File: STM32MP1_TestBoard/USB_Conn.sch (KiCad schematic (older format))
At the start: 4 parts, among them J13 USB_B_Micro, J14 USB_B

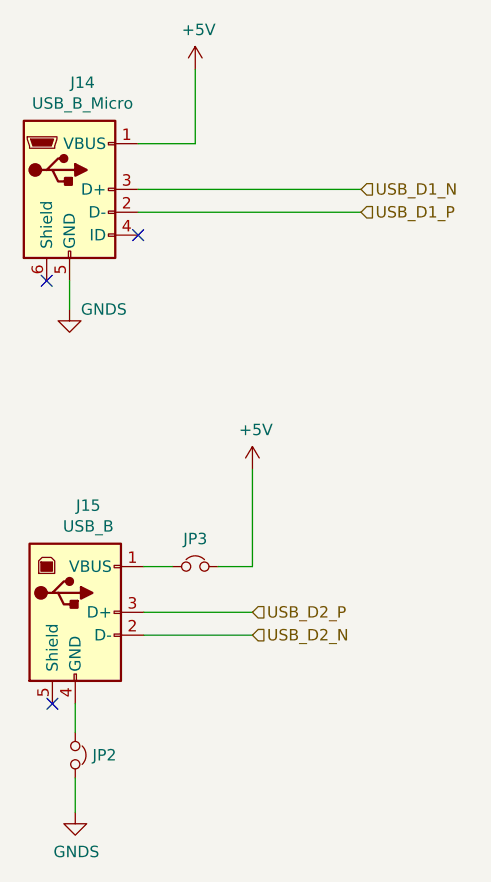
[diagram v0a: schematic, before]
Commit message: update
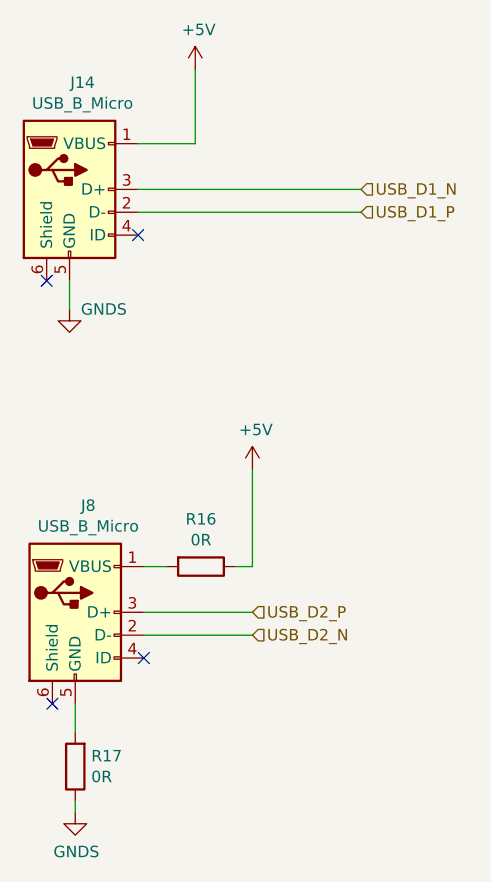
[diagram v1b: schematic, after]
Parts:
- removed J14: USB_B, Connector_USB:USB_B_Lumberg_2411_02_Horizontal, symbol Connector:USB_B
- removed JP2, JP3: Jumper_NC_Small, Jumper:SolderJumper-2_P1.3mm_Bridged_Pad1.0x1.5mm, symbol Device:Jumper_NC_Small
- added J8: USB_B_Micro, Connector_USB:USB_Micro-B_Molex-105017-0001, symbol Connector:USB_B_Micro
- added R16, R17: 0R, Resistor_SMD:R_0402_1005Metric_Pad0.72x0.64mm_HandSolder, symbol Device:R
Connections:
- net +5V: now also R16.1
- net GNDS: now also R17.1
- net USB_D2_N: now also J8.2 (D-)
- net USB_D2_P: now also J8.3 (D+)
- new net: J8.1 (VBUS), R16.2
- new net: J8.5 (GND), R17.2
- no-connect marks 3 -> 4
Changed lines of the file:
@@
 Wire Wire Line
 	4950 5150 5425 5150
-Wire Wire Line
-	4650 5450 4650 5575
 $Comp
 L power:GNDS #PWR0132
@@
 	1    0    0    -1
 $EndComp
-$Comp
-L Connector:USB_B J14
-U 1 1 5FC70F47
-P 4650 5050
-AR Path="/610FE7C3/5FC70F47" Ref="J14"  Part="1"
-AR Path="/6097C138/609989A6/5FC70F47" Ref="J15"  Part="1"
-F 0 "J15" H 4707 5517 50  0000 C CNN
-F 1 "USB_B" H 4707 5426 50  0000 C CNN
-F 2 "Connector_USB:USB_B_Lumberg_2411_02_Horizontal" H 4800 5000 50  0001 C CNN
-F 3 " ~" H 4800 5000 50  0001 C CNN
-	1    4650 5050
-	1    0    0    -1
-$EndComp
 Wire Wire Line
 	4925 3200 5900 3200
@@
 Wire Wire Line
 	4625 3600 4625 3725
-Wire Wire Line
-	4950 4850 5075 4850
 $Comp
-L Device:Jumper_NC_Small JP2
-U 1 1 5FC9168C
-P 5175 4850
-AR Path="/610FE7C3/5FC9168C" Ref="JP2"  Part="1"
-AR Path="/6097C138/609989A6/5FC9168C" Ref="JP3"  Part="1"
-F 0 "JP3" H 5175 4971 50  0000 C CNN
-F 1 "Jumper_NC_Small" H 5175 4971 50  0001 C CNN
-F 2 "Jumper:SolderJumper-2_P1.3mm_Bridged_Pad1.0x1.5mm" H 5175 4850 50  0001 C CNN
-F 3 "~" H 5175 4850 50  0001 C CNN
-	1    5175 4850
+L Connector:USB_B_Micro J?
+U 1 1 5FC689D6
+P 4650 5050
+AR Path="/610FE7C3/5FC689D6" Ref="J?"  Part="1"
+AR Path="/6097C138/609989A6/5FC689D6" Ref="J8"  Part="1"
+F 0 "J8" H 4707 5517 50  0000 C CNN
+F 1 "USB_B_Micro" H 4707 5426 50  0000 C CNN
+F 2 "Connector_USB:USB_Micro-B_Molex-105017-0001" H 4800 5000 50  0001 C CNN
+F 3 "~" H 4800 5000 50  0001 C CNN
+	1    4650 5050
 	1    0    0    -1
 $EndComp
+NoConn ~ 4950 5250
 Wire Wire Line
-	5275 4850 5425 4850
+	4950 4850 5050 4850
+Wire Wire Line
+	4650 5450 4650 5575
 $Comp
-L Device:Jumper_NC_Small JP3
-U 1 1 5FC94550
-P 4650 5675
-AR Path="/610FE7C3/5FC94550" Ref="JP3"  Part="1"
-AR Path="/6097C138/609989A6/5FC94550" Ref="JP2"  Part="1"
-F 0 "JP2" V 4650 5750 50  0000 L CNN
-F 1 "Jumper_NC_Small" H 4650 5796 50  0001 C CNN
-F 2 "Jumper:SolderJumper-2_P1.3mm_Bridged_Pad1.0x1.5mm" H 4650 5675 50  0001 C CNN
-F 3 "~" H 4650 5675 50  0001 C CNN
-	1    4650 5675
+L Device:R R16
+U 1 1 5FC7250A
+P 5200 4850
+F 0 "R16" V 4993 4850 50  0000 C CNN
+F 1 "0R" V 5084 4850 50  0000 C CNN
+F 2 "Resistor_SMD:R_0402_1005Metric_Pad0.72x0.64mm_HandSolder" V 5130 4850 50  0001 C CNN
+F 3 "~" H 5200 4850 50  0001 C CNN
+	1    5200 4850
 	0    1    1    0
 $EndComp
 Wire Wire Line
-	4650 5775 4650 5925
+	5350 4850 5425 4850
+$Comp
+L Device:R R17
+U 1 1 5FC752AF
+P 4650 5725
+F 0 "R17" H 4580 5679 50  0000 R CNN
+F 1 "0R" H 4580 5770 50  0000 R CNN
+F 2 "Resistor_SMD:R_0402_1005Metric_Pad0.72x0.64mm_HandSolder" V 4580 5725 50  0001 C CNN
+F 3 "~" H 4650 5725 50  0001 C CNN
+	1    4650 5725
+	-1   0    0    1
+$EndComp
+Wire Wire Line
+	4650 5875 4650 5925
 $EndSCHEMATC
